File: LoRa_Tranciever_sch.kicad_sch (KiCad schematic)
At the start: 16 parts, among them J3 Conn_Coaxial, U3 SX1280IMLTRT, Y1 52MHz

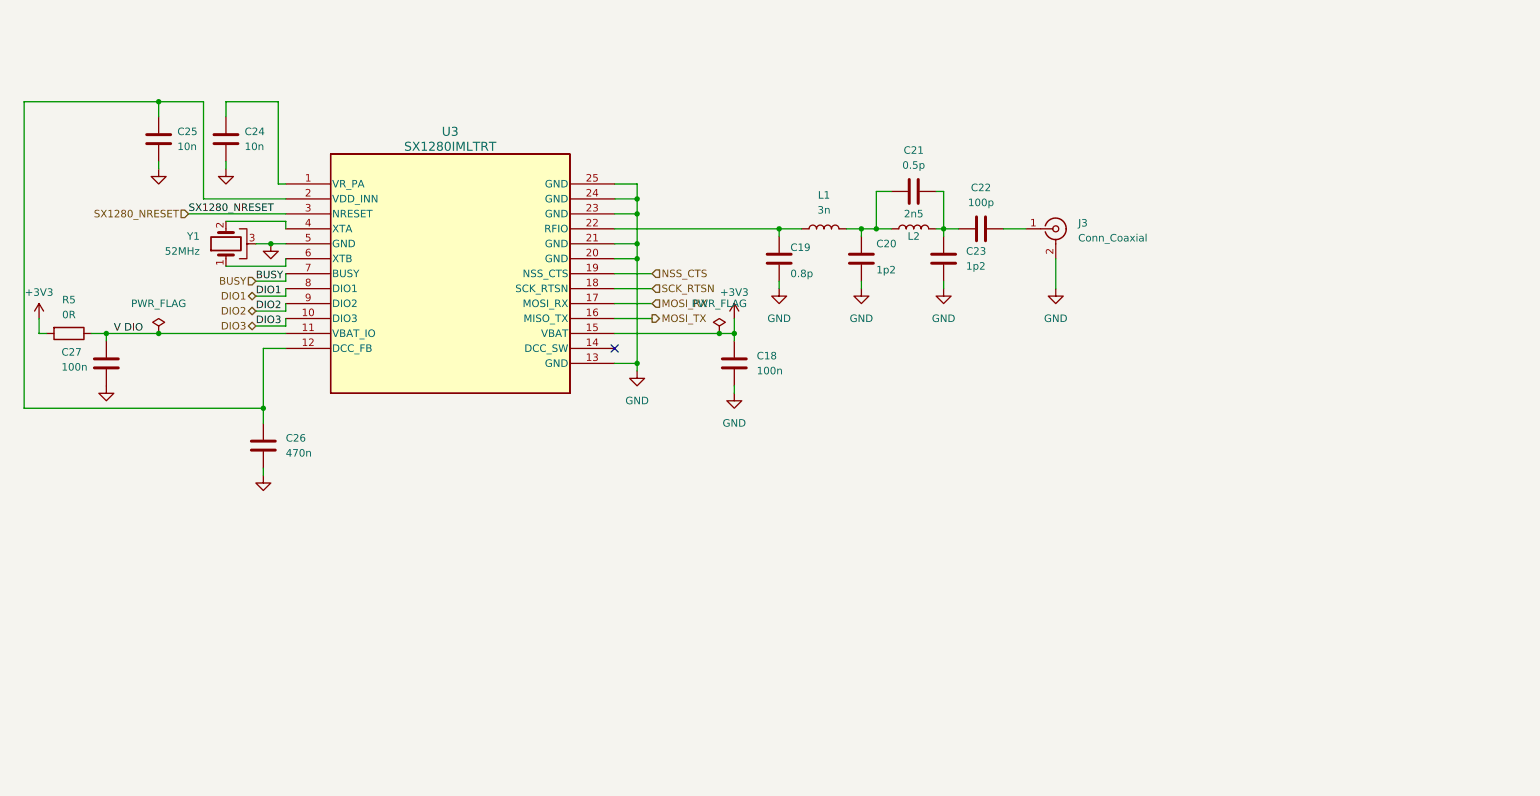
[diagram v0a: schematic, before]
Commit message: Done power
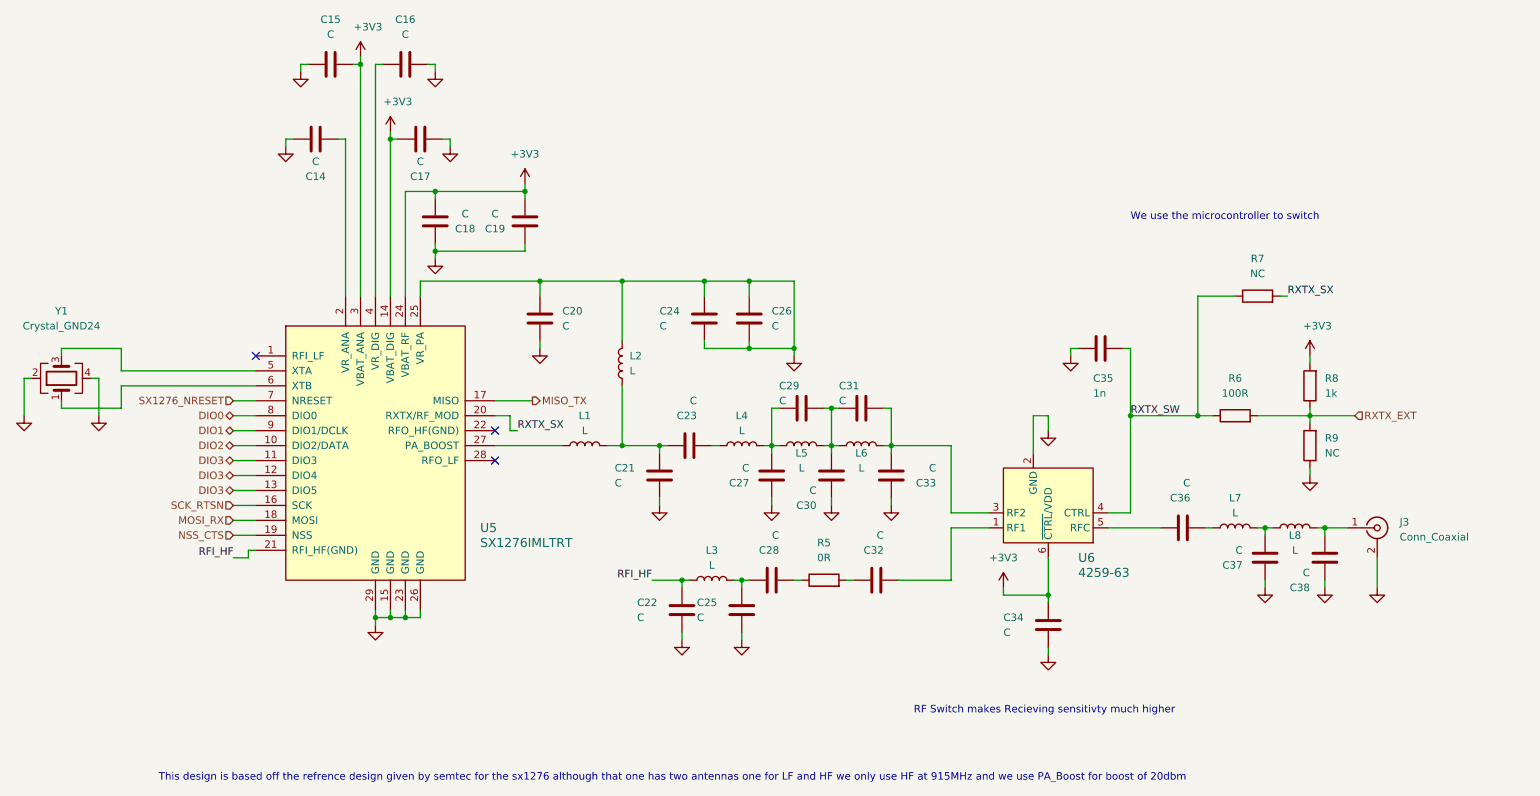
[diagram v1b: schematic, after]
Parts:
- removed U3: SX1280IMLTRT, footprints:QFN24_4X4_SEM, symbol RF_Parts:SX1280IMLTRT
- removed Y1: 52MHz, Crystal:Crystal_SMD_0603-4Pin_6.0x3.5mm, symbol Device:Crystal_GND3
- added C14, C15, C16, C17, C28, C29, C30, C31, C32, C33, C34, C36, C37, C38: C, symbol Device:C
- added C35: 1n, Capacitor_SMD:C_0402_1005Metric, symbol Device:C
- added L3, L4, L5, L6, L7, L8: L, symbol Device:L
- added R6: 100R, symbol Device:R
- added R7, R9: NC, symbol Device:R
- added R8: 1k, symbol Device:R
- added U5: SX1276IMLTRT, digikey-footprints:VQFN-28-1EP_6x6mm, symbol dk_RF-Transceiver-ICs:SX1276IMLTRT
- added U6: 4259-63, digikey-footprints:SOT-363, symbol dk_RF-Switches:4259-63
- added Y1: Crystal_GND24, symbol Device:Crystal_GND24
- C18, C27: value 100n -> C; footprint Capacitor_SMD:C_0402_1005Metric -> (none)
- C19: value 0.8p -> C; footprint Capacitor_SMD:C_0402_1005Metric -> (none)
- C20, C23: value 1p2 -> C; footprint Capacitor_SMD:C_0402_1005Metric -> (none)
- C21: value 0.5p -> C; footprint Capacitor_SMD:C_0402_1005Metric -> (none)
- C22: value 100p -> C; footprint Capacitor_SMD:C_0402_1005Metric -> (none)
- C24, C25: value 10n -> C; footprint Capacitor_SMD:C_0402_1005Metric -> (none)
- C26: value 470n -> C; footprint Capacitor_SMD:C_0402_1005Metric -> (none)
- J3: footprint footprints:TAOGLAS_EMPCB.SMAFSTJ.B.HT -> Connector_Coaxial:SMA_Amphenol_132289_EdgeMount; JLC # (none) -> C2987684
- L1: value 3n -> L; footprint Inductor_SMD:L_0402_1005Metric -> (none)
- L2: value 2n5 -> L; footprint Inductor_SMD:L_0402_1005Metric -> (none)
- R5: footprint Capacitor_SMD:C_0402_1005Metric -> (none)
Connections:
- net +3V3: now also C19.1, C15.1, C17.1, C34.1, R8.2, U5.14 (VBAT_DIG), U5.24 (VBAT_RF), U5.3 (VBAT_ANA), U6.6 (~{CTRL}/VDD); no longer R5.2
- net DIO1: now also U5.9 (DIO1/DCLK)
- net DIO2: now also U5.10 (DIO2/DATA)
- net DIO3: now also U5.11 (DIO3), U5.12 (DIO4), U5.13 (DIO5)
- net GND: now also C19.2, C20.1, C21.2, C22.2, C24.1, C26.1, C27.1, L2.2, C14.2, C15.2, C16.2, C17.2, C30.1, C33.1, C34.2, C35.2, C37.1, C38.1, R9.1, U5.15 (GND), U5.23 (GND), U5.25 (VR_PA), U5.26 (GND), U5.29 (GND), U6.2 (GND), Y1.2, Y1.4; no longer C19.1, C23.1, C27.2
- net MOSI_RX: now also U5.18 (MOSI)
- net NSS_CTS: now also U5.19 (NSS)
- net SCK_RTSN: now also U5.16 (SCK)
- net at C25.1: now also C28.1, L3.2; no longer C26.1
- net at J3.1 (In): now also C38.2, L8.2; no longer C22.2
- net at C21.1, L1.2, L2.1: now also C23.1; no longer C20.1
- net at L1.1: now also U5.27 (PA_BOOST); no longer C19.2
- net V DIO: no longer names the net of R5.1
- net V DIO: now also C28.2; no longer C27.1
- new net: C37.2, L7.2, L8.1
- new net: C16.1, U5.4 (VR_DIG)
- new net: C23.2, L4.1
- new net: C27.2, C29.2, L4.2, L5.1
- new net: C29.1, C30.2, C31.2, L5.2, L6.1
- new net: C31.1, C33.2, L6.2, U6.3 (RF2)
- new net: C14.1, U5.2 (VR_ANA)
- new net: U5.5 (XTA), Y1.3
- new net: U5.6 (XTB), Y1.1
- new net: C32.1, R5.2
- new net: C32.2, U6.1 (RF1)
- new net: C36.1, U6.5 (RFC)
- new net: C36.2, L7.1
- new net DIO0: U5.8 (DIO0)
- new net MISO_TX: U5.17 (MISO)
- new net RFI_HF: C22.1, L3.1, U5.21 (RFI_HF(GND))
- new net RXTX_EXT: R6.2, R8.1, R9.2
- new net RXTX_SW: C35.1, R6.1, R7.1, U6.4 (CTRL)
- new net RXTX_SX: R7.2, U5.20 (RXTX/RF_MOD)
- new net SX1276_NRESET: U5.7 (NRESET)
- no-connect marks 1 -> 3
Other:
- note added: "RF Switch makes Recieving sensitivty much higher"
- note added: "This design is based off the refrence design given by semtec for the sx1276 although that one has two antennas one for LF and HF we only use HF at 915MHz and we use PA_Boost for boost of 20dbm"
- note added: "We use the microcontroller to switch"
